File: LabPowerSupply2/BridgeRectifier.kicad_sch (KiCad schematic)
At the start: 6 parts

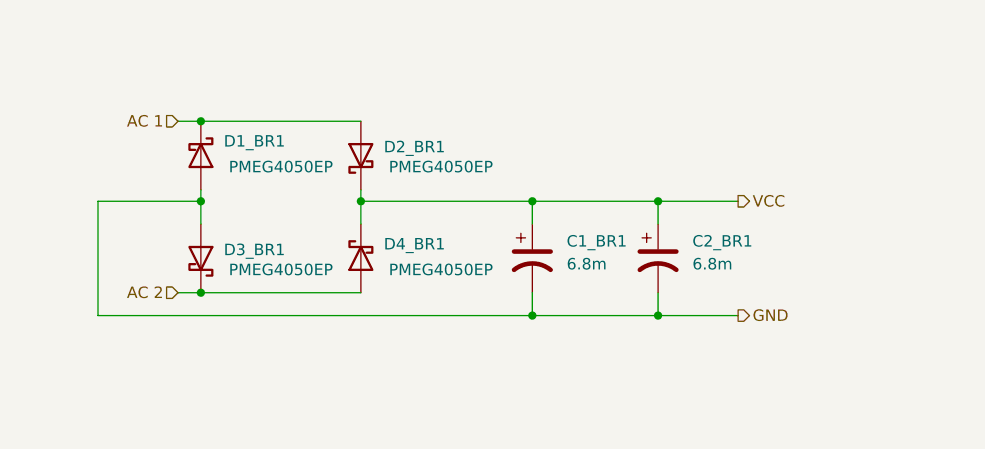
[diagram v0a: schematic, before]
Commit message: Beautifing the Schematic
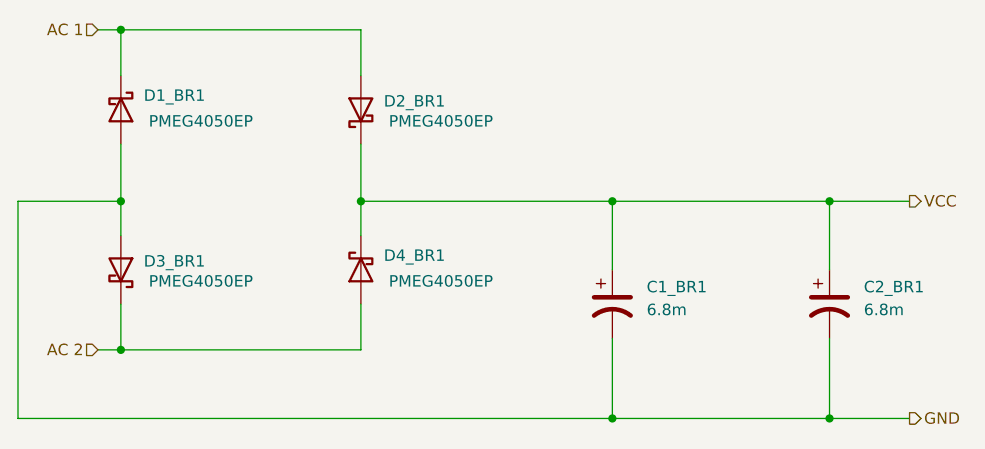
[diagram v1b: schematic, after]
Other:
- moved on the sheet: C1_BR1, C2_BR1, D1_BR1, D2_BR1, D3_BR1, D4_BR1
